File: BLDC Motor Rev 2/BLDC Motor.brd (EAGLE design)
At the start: 60.6 x 67 mm, 53 parts, among them IC1 7805TV, IC2 7815TV, Q1 TP2104, Q10 TP2104, Q12 IRFS, Q13 TP2104, Q15 IRFS, Q16 TP2104, Q18 IRFS, Q3 IRFS, Q4 TP2104, Q6 IRFS, Q7 TP2104, Q9 IRFS, U1 ATMEGA328P_TQFP, Y1 16M

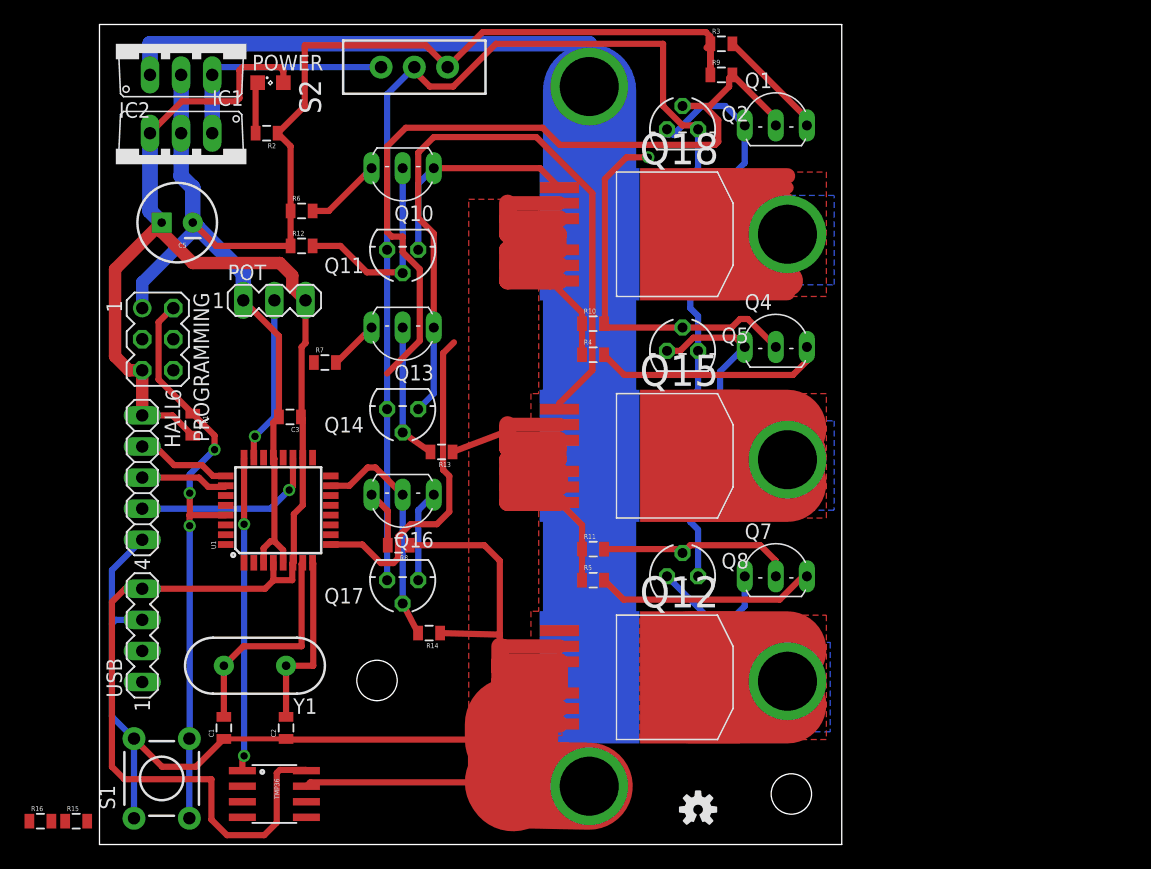
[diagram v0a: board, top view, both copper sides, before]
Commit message: Updating board
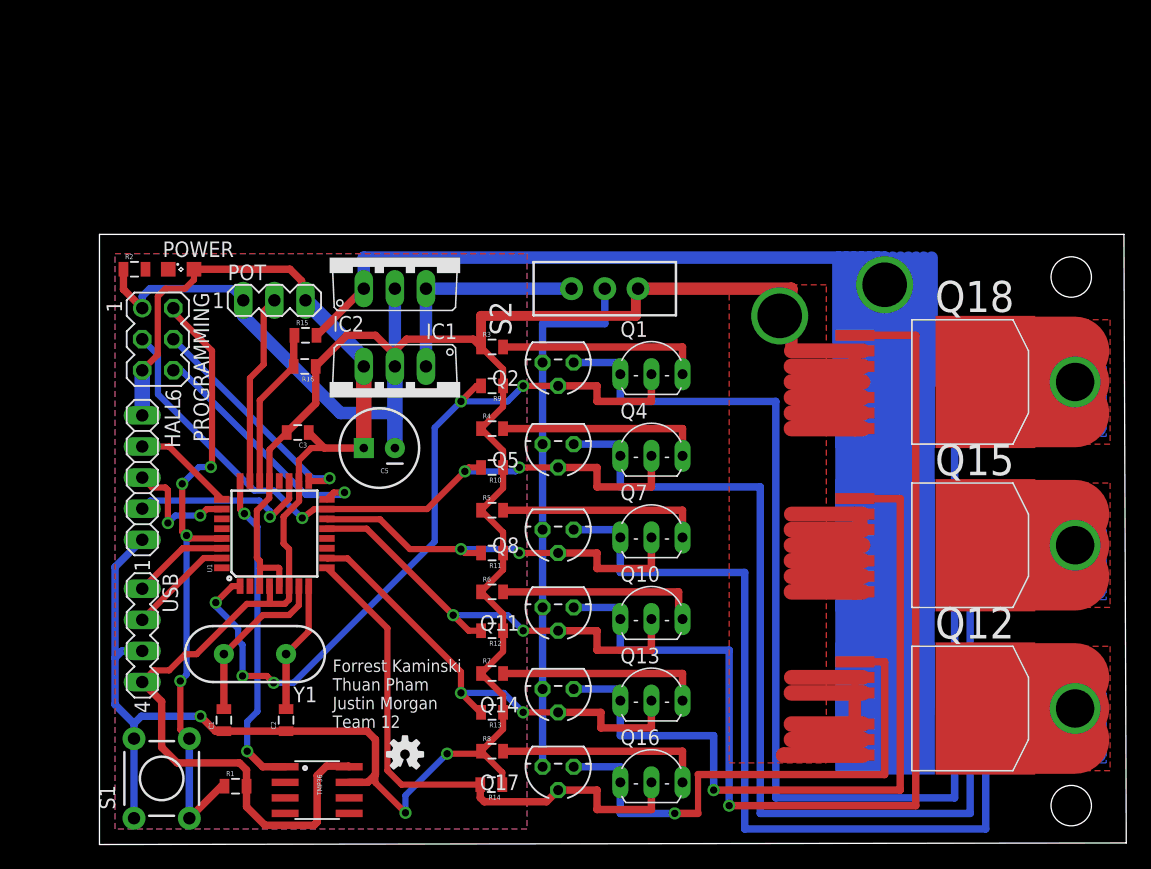
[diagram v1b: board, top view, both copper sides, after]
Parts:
- removed JP4: STAND-OFF, SparkFun:STAND-OFF
- added JP1: STAND-OFF, SparkFun:STAND-OFF
- R16: value 20k -> 22k
- moved JP2 57.6 mm to (79.4, 3.17)
- moved R15 43.9 mm to (16.8, 41.6)
- moved R16 43.0 mm to (16.8, 39.1), turned to 180 degrees
- moved Q10 42.1 mm to (45.1, 18.4), turned to 0 degrees
- moved Q13 36.6 mm to (45.1, 11.7), turned to 0 degrees
- moved R12 35.1 mm to (32.1, 17.5), turned to 180 degrees
- moved R6 34.8 mm to (32.1, 20.6)
- moved Q11 31.9 mm to (37.5, 19.4)
- moved R9 31.6 mm to (32.1, 37.5), turned to 180 degrees
- moved Q16 31.1 mm to (45.1, 5.08), turned to 0 degrees
- moved R3 31.1 mm to (32.1, 40.6)
- moved R1 29.7 mm to (11.1, 4.76), turned to 0 degrees
- moved R7 28.8 mm to (32.1, 14.0)
- moved Q18 27.0 mm to (68.3, 37.8)
- moved Q3 27.0 mm to (68.3, 37.8)
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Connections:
- net MOSI: now also Q4.2, Q5.2, R10.2; no longer Q16.2, Q17.2, R14.2
- net PULSE2: now also Q16.2, Q17.2, R14.2; no longer Q4.2, Q5.2, R10.2
- net PULSE3: now also Q13.2, Q14.2, R13.2; no longer Q7.2, Q8.2, R11.2
- net PULSE5: now also Q7.2, Q8.2, R11.2; no longer Q13.2, Q14.2, R13.2
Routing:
- net BATTPOS: track 90.2 -> 209.3 mm
- net N$5: track 13.9 -> 109.4 mm
- net N$13: track 13.0 -> 92.0 mm
- net N$19: track 18.1 -> 87.5 mm, vias 0 -> 1
- net N$9: track 111.7 -> 44.1 mm
- net N$16: track 11.5 -> 74.2 mm
- net PHASEA: track 116.4 -> 69.0 mm
- net MOSI: track 19.0 -> 56.7 mm, vias 0 -> 3
- net N$25: track 7.51 -> 44.0 mm, vias 0 -> 1
- net VCC: track 140.9 -> 105.4 mm
- net PULSE3: track 16.2 -> 38.5 mm, vias 0 -> 2
- net PULSE5: track 11.3 -> 33.2 mm, vias 0 -> 2
- net PULSE4: track 16.8 -> 36.9 mm, vias 0 -> 2
- net MISO: track 0.00 -> 19.9 mm, vias 0 -> 1
- net SCK: track 0.00 -> 19.3 mm, vias 0 -> 1
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- added copper zone on layer 16, net BATTPOS
- added copper zone on layer 16, net GND
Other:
- board size 60.6 x 67 mm -> 83.9 x 49.8 mm
- board text added: "Forrest Kaminski Thuan Pham Justin Morgan Team 12"
